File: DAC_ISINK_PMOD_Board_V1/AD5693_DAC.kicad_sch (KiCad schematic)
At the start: 10 parts, among them U1 AD5691RxRM

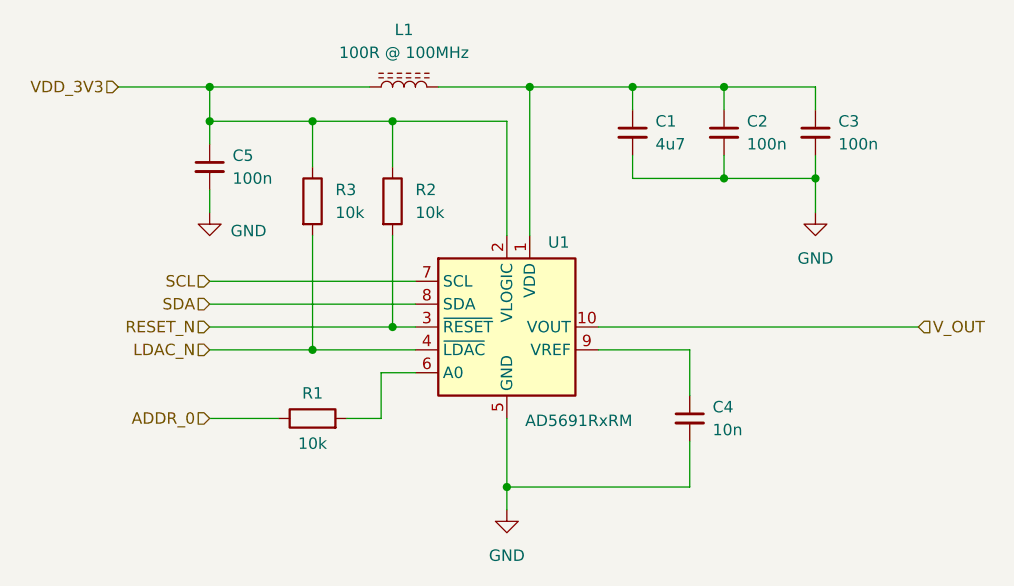
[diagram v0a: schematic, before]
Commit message: Manufacturing Data Generated.
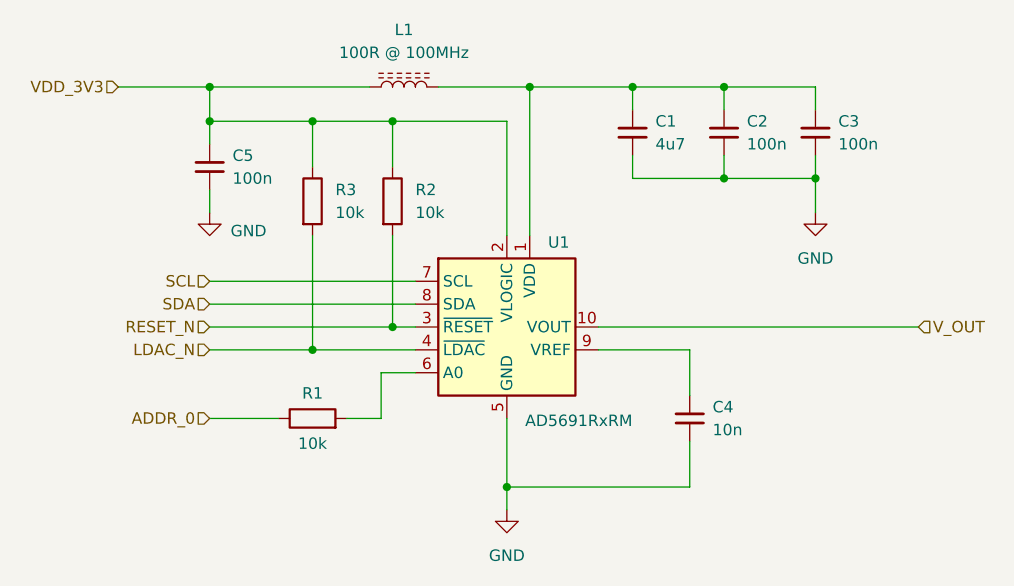
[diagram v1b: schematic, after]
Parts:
- C1, C2, C3, C4, C5: footprint (none) -> Capacitor_SMD:C_0603_1608Metric
- L1: footprint (none) -> Inductor_SMD:L_0603_1608Metric
- R1, R2, R3: footprint (none) -> Resistor_SMD:R_0603_1608Metric
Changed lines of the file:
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@@
 			)
 		)
-		(property "Footprint" ""
+		(property "Footprint" "Resistor_SMD:R_0603_1608Metric"
 			(at 130.302 52.07 90)
 			(hide yes)
@@
 			)
 		)
-		(property "Footprint" ""
+		(property "Footprint" "Capacitor_SMD:C_0603_1608Metric"
 			(at 179.07 44.45 0)
 			(hide yes)
@@
 			)
 		)
-		(property "Footprint" ""
+		(property "Footprint" "Capacitor_SMD:C_0603_1608Metric"
 			(at 165.1 76.2 0)
 			(hide yes)
@@
 			)
 		)
-		(property "Footprint" ""
+		(property "Footprint" "Capacitor_SMD:C_0603_1608Metric"
 			(at 158.75 44.45 0)
 			(hide yes)
@@
 			)
 		)
-		(property "Footprint" ""
+		(property "Footprint" "Capacitor_SMD:C_0603_1608Metric"
 			(at 111.76 48.26 0)
 			(hide yes)
@@
 			)
 		)
-		(property "Footprint" ""
+		(property "Footprint" "Resistor_SMD:R_0603_1608Metric"
 			(at 123.19 77.978 90)
 			(hide yes)
@@
 			)
 		)
-		(property "Footprint" ""
+		(property "Footprint" "Inductor_SMD:L_0603_1608Metric"
 			(at 133.35 39.37 0)
 			(hide yes)
@@
 			)
 		)
-		(property "Footprint" ""
+		(property "Footprint" "Resistor_SMD:R_0603_1608Metric"
 			(at 121.412 52.07 90)
 			(hide yes)
@@
 			)
 		)
-		(property "Footprint" ""
+		(property "Footprint" "Capacitor_SMD:C_0603_1608Metric"
 			(at 168.91 44.45 0)
 			(hide yes)
